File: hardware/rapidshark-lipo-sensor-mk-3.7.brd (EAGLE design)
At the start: 33 x 17.8 mm, 32 parts, among them Q1 BSH203, Q2 MMBT2222A, Q3 BSH203, Q4 MMBT2222A, Q5 BSH203, Q6 MMBT2222A, U1 Tiny84

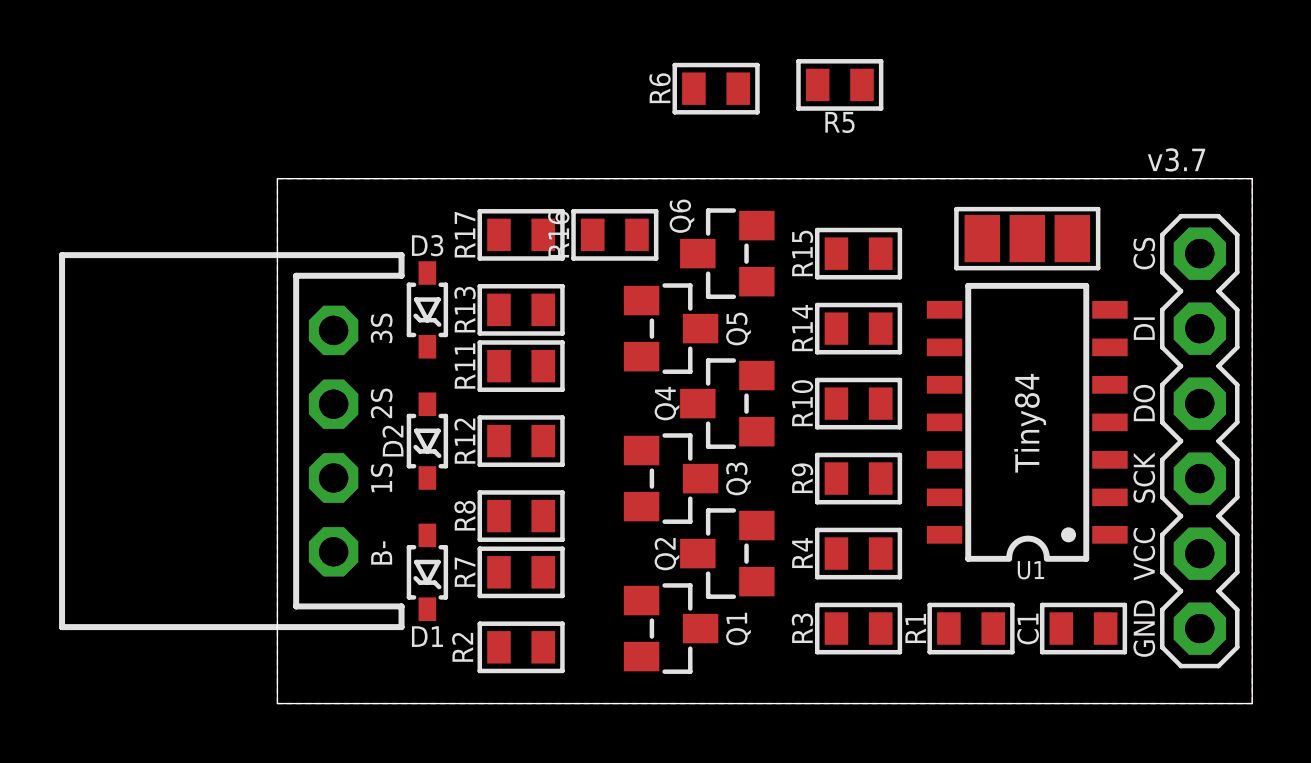
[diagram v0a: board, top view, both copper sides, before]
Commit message: oh hey more hardware fails
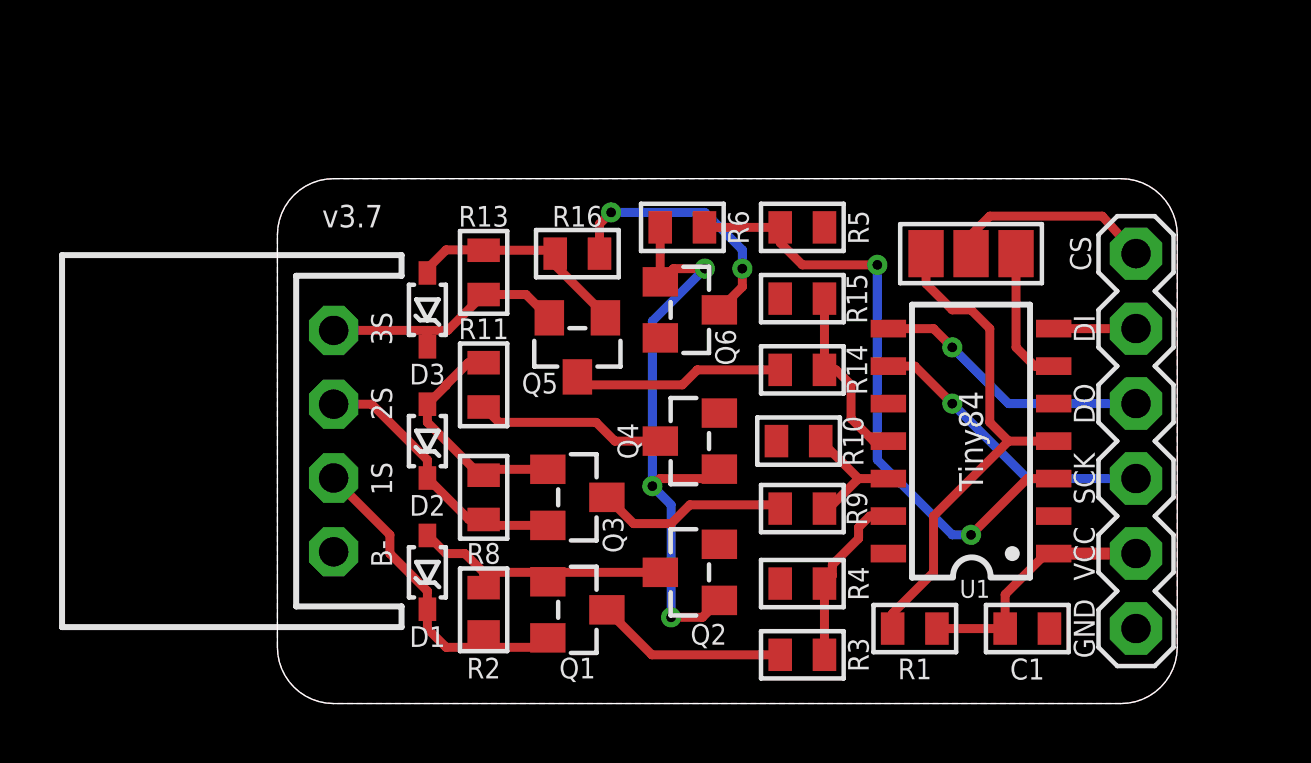
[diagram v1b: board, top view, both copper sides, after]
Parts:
- removed R12, R17, R7: 100R, a_parts:R0603-TIGHTER
- moved R5 4.99 mm to (17.8, 16.1)
- moved R6 4.84 mm to (13.7, 16.1)
- moved Q1 3.24 mm to (10.2, 3.17)
- moved Q3 3.24 mm to (10.2, 6.99)
- moved Q5 3.24 mm to (10.2, 12.1), turned to 180 degrees
- moved R15 2.44 mm to (17.8, 13.7)
- moved R10 2.40 mm to (17.7, 8.89)
- moved R14 2.36 mm to (17.8, 11.3)
- moved Q6 2.29 mm to (14.0, 13.3), turned to 270 degrees
- moved JP2 2.16 mm to (29.1, 8.89)
- moved R4 2.16 mm to (17.8, 4.06)
- moved R9 2.16 mm to (17.8, 6.60)
- moved R3 2.10 mm to (17.8, 1.65)
- moved U1 2.01 mm to (23.5, 8.89)
- moved RST/CS 1.97 mm to (23.5, 15.2)
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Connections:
- removed net N$10: Q1.1, R7.1
- removed net N$11: Q3.1, R12.1
- removed net N$12: Q5.1, R17.1
- net N$5: now also Q3.1; no longer R12.2
- net N$7: now also Q5.1; no longer R17.2
- net N$9: now also Q1.1; no longer R7.2
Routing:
- net EN_DIV: track 0.00 -> 21.1 mm, vias 0 -> 2
- net EN_DIV_RLY: track 0.00 -> 20.7 mm, vias 0 -> 3
- net RESET: track 0.00 -> 17.4 mm
- net CELL1+: track 0.00 -> 11.4 mm
- net SCK: track 0.00 -> 9.97 mm, vias 0 -> 1
- net DO/MISO: track 0.00 -> 9.44 mm, vias 0 -> 1
- net CELL2+: track 0.00 -> 9.32 mm
- net N$9: track 0.00 -> 9.19 mm
- net N$8: track 0.00 -> 8.89 mm, vias 0 -> 2
- net CELL3+: track 0.00 -> 8.69 mm
- net VCC: track 0.00 -> 8.47 mm
- net N$5: track 0.00 -> 8.05 mm
- net N$7: track 0.00 -> 7.67 mm
- net N$3: track 0.00 -> 7.19 mm
- net RST/CS: track 0.00 -> 7.05 mm
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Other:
- board size 33 x 17.8 mm -> 30.5 x 17.8 mm
